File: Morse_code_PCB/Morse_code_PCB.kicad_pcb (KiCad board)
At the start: 2 copper layers, 60 x 30 mm, 66 parts, among them J1 USB_C_Receptacle_USB2.0, J2 INPUT, J3 OUTPUT, J4 Conn_01x02_Female, J5 Conn_01x04_Female, Q1 AO3400A, Q2 AO3401A, Q3 AO3400A, Q4 AO3401A, SW1 RotaryEncoder_Switch, U1 STM32F030F4Px, U2 OLED_12864, U3 MCP73831-2-OT, U4 CH340E, U5 LP5907MFX-3.3, U6 24AA02-OT, U7 STM32F103C8Tx, Y1 8M, Y2 32.768k

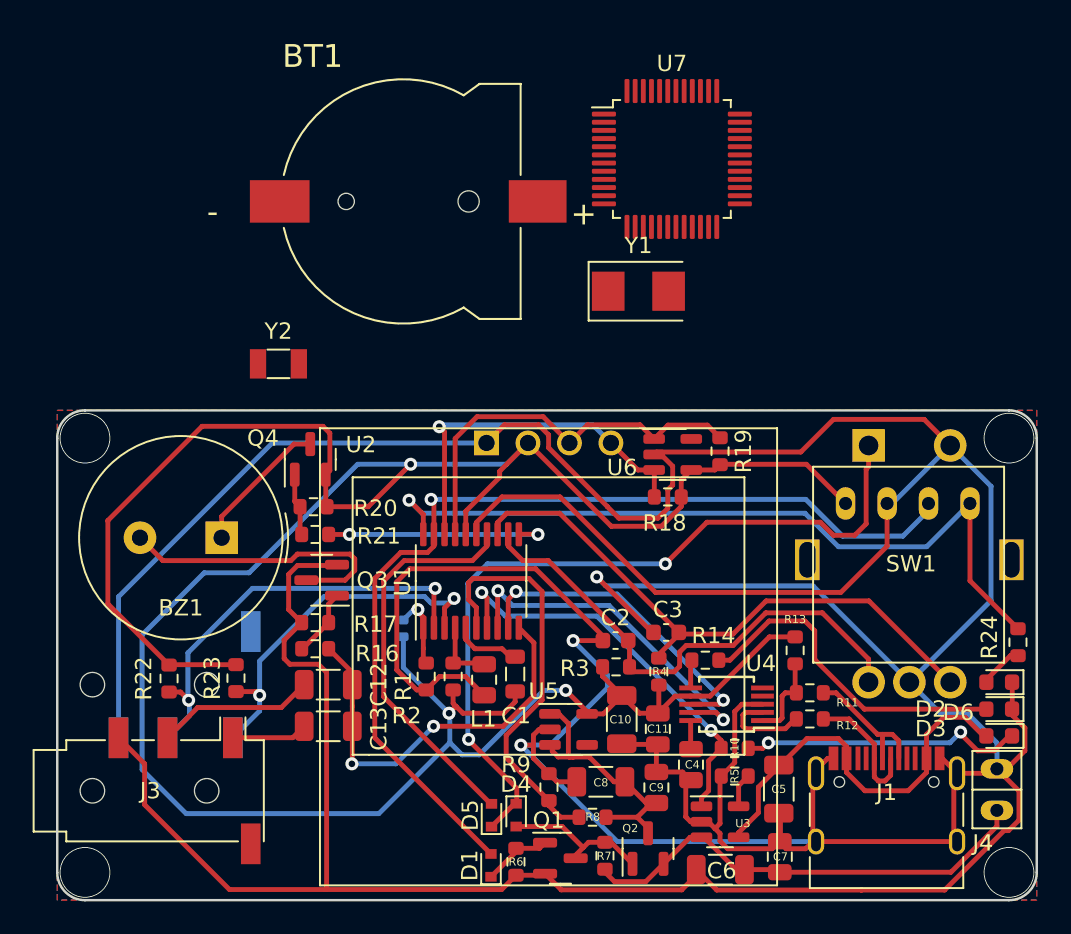
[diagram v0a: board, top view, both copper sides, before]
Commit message: Updata PCB Signed-off-by: kevin <kevin@lmve.net>
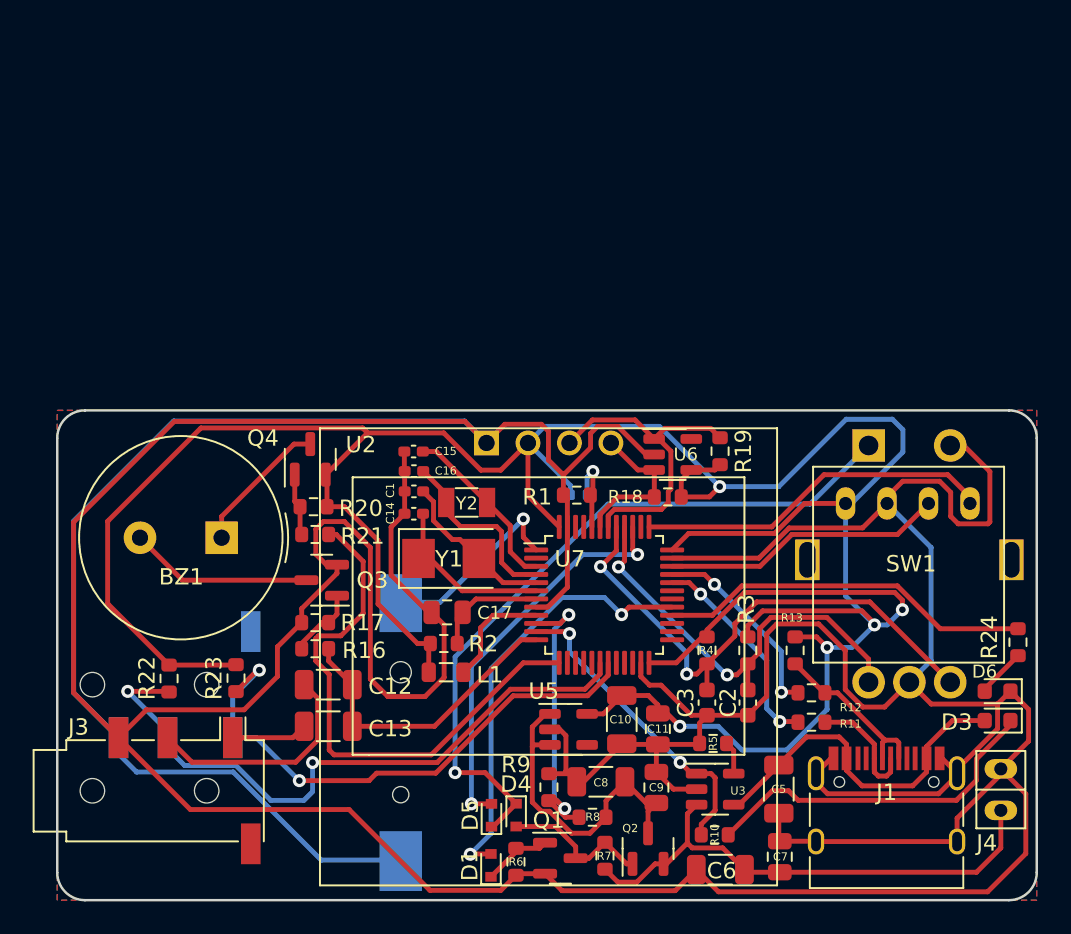
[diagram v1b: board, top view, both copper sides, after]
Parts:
- removed C4: 104, Capacitor_SMD:C_0805_2012Metric
- removed D2: LED, LED_SMD:LED_0603_1608Metric
- removed R14: 510, Resistor_SMD:R_0603_1608Metric
- removed U1: STM32F030F4Px, Package_SO:TSSOP-20_4.4x6.5mm_P0.65mm
- removed U4: CH340E, Package_SO:MSOP-10_3x3mm_P0.5mm
- removed https://git.lmve.net/summary/~kevin%2FMorse_code_trainer.git: LOGO, MY:code
- added C14: C, Capacitor_SMD:C_0402_1005Metric_Pad0.74x0.62mm_HandSolder, F.Cu at (91.8, 138.3)
- added C15: C, Capacitor_SMD:C_0402_1005Metric_Pad0.74x0.62mm_HandSolder, F.Cu at (91.8, 134.5)
- added C16: C, Capacitor_SMD:C_0402_1005Metric_Pad0.74x0.62mm_HandSolder, F.Cu at (91.8, 135.7)
- added C17: 100nF, Capacitor_SMD:C_0805_2012Metric, F.Cu at (93.9, 144.4)
- BT1: moved to B.Cu
- C1: value 100nF -> C; footprint Capacitor_SMD:C_0805_2012Metric -> Capacitor_SMD:C_0402_1005Metric_Pad0.74x0.62mm_HandSolder
- moved BT1 32.8 mm to (91.0, 152.0), turned to 90 degrees
- moved U7 27.0 mm to (103.5, 143.3)
- moved Y1 20.1 mm to (94.0, 141.1)
- moved R1 14.4 mm to (101.8, 137.2), turned to 0 degrees
- moved Y2 14.3 mm to (95.1, 137.6), turned to 180 degrees
- moved R15 13.5 mm to (102.0, 137.2), turned to 0 degrees
- moved C1 12.3 mm to (91.8, 137.0), turned to 0 degrees
- moved C2 8.95 mm to (112.3, 149.9), turned to -90 degrees
- moved R3 8.13 mm to (112.3, 146.7), turned to 90 degrees
- moved R10 5.44 mm to (110.3, 158.0)
- moved C3 4.97 mm to (109.8, 149.9), turned to -90 degrees
- moved L1 4.23 mm to (93.8, 148.0), turned to 0 degrees
- moved R4 3.22 mm to (109.8, 146.7), turned to 90 degrees
- moved R5 2.40 mm to (110.2, 152.4)
- moved R2 2.10 mm to (93.7, 146.3), turned to 180 degrees
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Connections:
- BT1 pad 1: unconnected-(BT1-Pad1) -> Net-(BT1-Pad1)
- BT1 pad 2: unconnected-(BT1-Pad2) -> GND
- C1 pad 1: Net-(C1-Pad1) -> GND
- C1 pad 2: GND -> Net-(U7-Pad5)
- C2 pad 1: Net-(C2-Pad1) -> EN_A
- C3 pad 1: Net-(C3-Pad1) -> EN_B
- J1 pad A6: Net-(J1-PadA6) -> Net-(R13-Pad1)
- J1 pad A7: Net-(J1-PadA7) -> Net-(R11-Pad2)
- J1 pad B6: Net-(J1-PadA6) -> Net-(R13-Pad1)
- J1 pad B7: Net-(J1-PadA7) -> Net-(R11-Pad2)
- J5 pad 3: PWR_EN -> SW_D
- J5 pad 4: RUN_LED -> SW_L
- L1 pad 2: Net-(L1-Pad2) -> Net-(U7-Pad9)
- R1 pad 2: Net-(R1-Pad2) -> Net-(U7-Pad44)
- R11 pad 1: Net-(R11-Pad1) -> USB_DN
- R11 pad 2: Net-(J1-PadA6) -> Net-(R11-Pad2)
- R12 pad 1: Net-(R12-Pad1) -> USB_DP
- R12 pad 2: Net-(J1-PadA7) -> Net-(R13-Pad1)
- R13 pad 1: VCC -> Net-(R13-Pad1)
- R13 pad 2: Net-(R11-Pad1) -> VCC
- R15 pad 2: Net-(R1-Pad2) -> Net-(U7-Pad44)
- R2 pad 1: Net-(C1-Pad1) -> Net-(U7-Pad7)
- R3 pad 1: Net-(C2-Pad1) -> EN_A
- R4 pad 1: Net-(C3-Pad1) -> EN_B
- SW1 pad A: Net-(C2-Pad1) -> EN_A
- SW1 pad B: Net-(C3-Pad1) -> EN_B
- U7 pad 1: unconnected-(U7-Pad1) -> Net-(BT1-Pad1)
- U7 pad 10: unconnected-(U7-Pad10) -> BAT_ADC
- U7 pad 11: unconnected-(U7-Pad11) -> BAT_CHG_DET
- U7 pad 12: unconnected-(U7-Pad12) -> PWM
- U7 pad 13: unconnected-(U7-Pad13) -> MUTE
- U7 pad 18: unconnected-(U7-Pad18) -> TICK_A
- U7 pad 19: unconnected-(U7-Pad19) -> TICK_B
- U7 pad 23: unconnected-(U7-Pad23) -> GND
- U7 pad 24: unconnected-(U7-Pad24) -> VCC
- U7 pad 28: unconnected-(U7-Pad28) -> RUN_LED
- U7 pad 29: unconnected-(U7-Pad29) -> PWR_EN
- U7 pad 3: unconnected-(U7-Pad3) -> Net-(U7-Pad3)
- U7 pad 30: unconnected-(U7-Pad30) -> RXD
- U7 pad 31: unconnected-(U7-Pad31) -> TXD
- U7 pad 32: unconnected-(U7-Pad32) -> USB_DN
- U7 pad 33: unconnected-(U7-Pad33) -> USB_DP
- U7 pad 34: unconnected-(U7-Pad34) -> SW_D
- U7 pad 35: unconnected-(U7-Pad35) -> GND
- U7 pad 36: unconnected-(U7-Pad36) -> VCC
- U7 pad 37: unconnected-(U7-Pad37) -> SW_L
- U7 pad 39: unconnected-(U7-Pad39) -> K1_DET
- U7 pad 4: unconnected-(U7-Pad4) -> Net-(U7-Pad4)
- U7 pad 40: unconnected-(U7-Pad40) -> EN_A
- U7 pad 41: unconnected-(U7-Pad41) -> EN_B
- U7 pad 42: unconnected-(U7-Pad42) -> IIC_SCL
- U7 pad 43: unconnected-(U7-Pad43) -> IIC_SDL
- U7 pad 44: unconnected-(U7-Pad44) -> Net-(U7-Pad44)
- U7 pad 47: unconnected-(U7-Pad47) -> GND
- U7 pad 48: unconnected-(U7-Pad48) -> VCC
- U7 pad 5: unconnected-(U7-Pad5) -> Net-(U7-Pad5)
- U7 pad 6: unconnected-(U7-Pad6) -> Net-(U7-Pad6)
- U7 pad 7: unconnected-(U7-Pad7) -> Net-(U7-Pad7)
- U7 pad 8: unconnected-(U7-Pad8) -> GND
- U7 pad 9: unconnected-(U7-Pad9) -> Net-(U7-Pad9)
- Y1 pad 1: unconnected-(Y1-Pad1) -> Net-(U7-Pad6)
- Y1 pad 2: unconnected-(Y1-Pad2) -> Net-(U7-Pad5)
- Y2 pad 1: unconnected-(Y2-Pad1) -> Net-(U7-Pad4)
- Y2 pad 2: unconnected-(Y2-Pad2) -> Net-(U7-Pad3)
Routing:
- net Net-(C3-Pad1): track 36.7 -> 0.00 mm
- net EN_B: track 0.00 -> 33.7 mm, vias 0 -> 2
- net PWR_EN: track 59.7 -> 26.7 mm, vias 1 -> 2
- net Net-(C2-Pad1): track 31.5 -> 0.00 mm
- net EN_A: track 0.00 -> 27.0 mm, vias 0 -> 2
- net RUN_LED: track 48.0 -> 23.0 mm, vias 1 -> 0
- net SW_L: track 0.00 -> 21.9 mm
- net RXD: track 21.5 -> 0.00 mm, vias 2 -> 0
- net Net-(D2-Pad2): track 20.5 -> 0.00 mm
- net TXD: track 20.0 -> 0.00 mm, vias 2 -> 0
- net MUTE: track 14.0 -> 33.2 mm, vias 2 -> 0
- net SW_D: track 0.00 -> 17.3 mm
- net VCC: track 177.0 -> 190.6 mm, vias 3 -> 5
- net TICK_A: track 26.4 -> 39.8 mm
- net IIC_SDL: track 22.7 -> 9.52 mm, vias 1 -> 0
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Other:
- board text added: "Morse code practice V2 Designed by Kevin 2022-4-9"
- board text added: "https://git.lmve.net/kevin/morse_code_trainer"
- board text removed: "Morse code practice Designed by Kevin 2022-3-18"
